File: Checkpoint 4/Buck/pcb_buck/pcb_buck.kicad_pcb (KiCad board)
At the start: 2 copper layers, 90.2 x 37.8 mm, 18 parts, among them J2 Conn_01x04_Socket, M1 IRF530, M2 IRF530, U1 IR2104

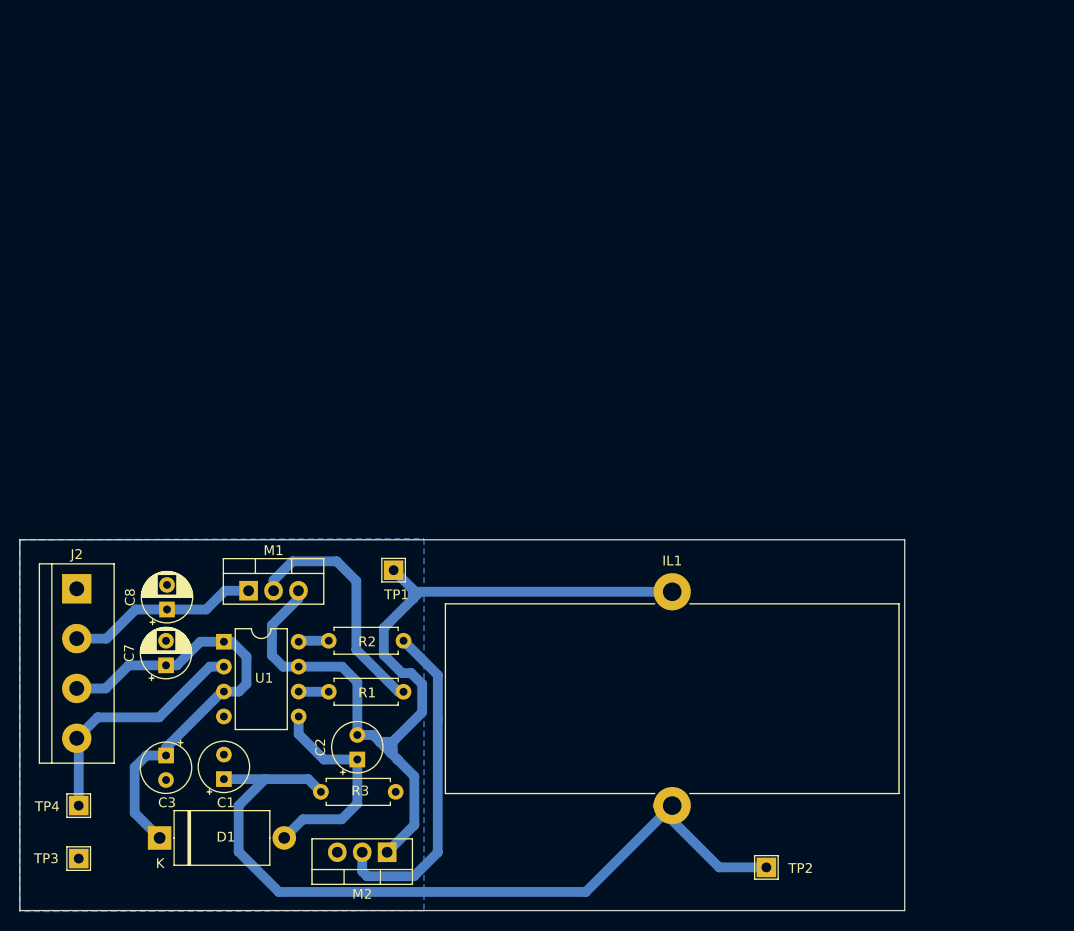
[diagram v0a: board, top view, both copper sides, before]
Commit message: PCB Buck new
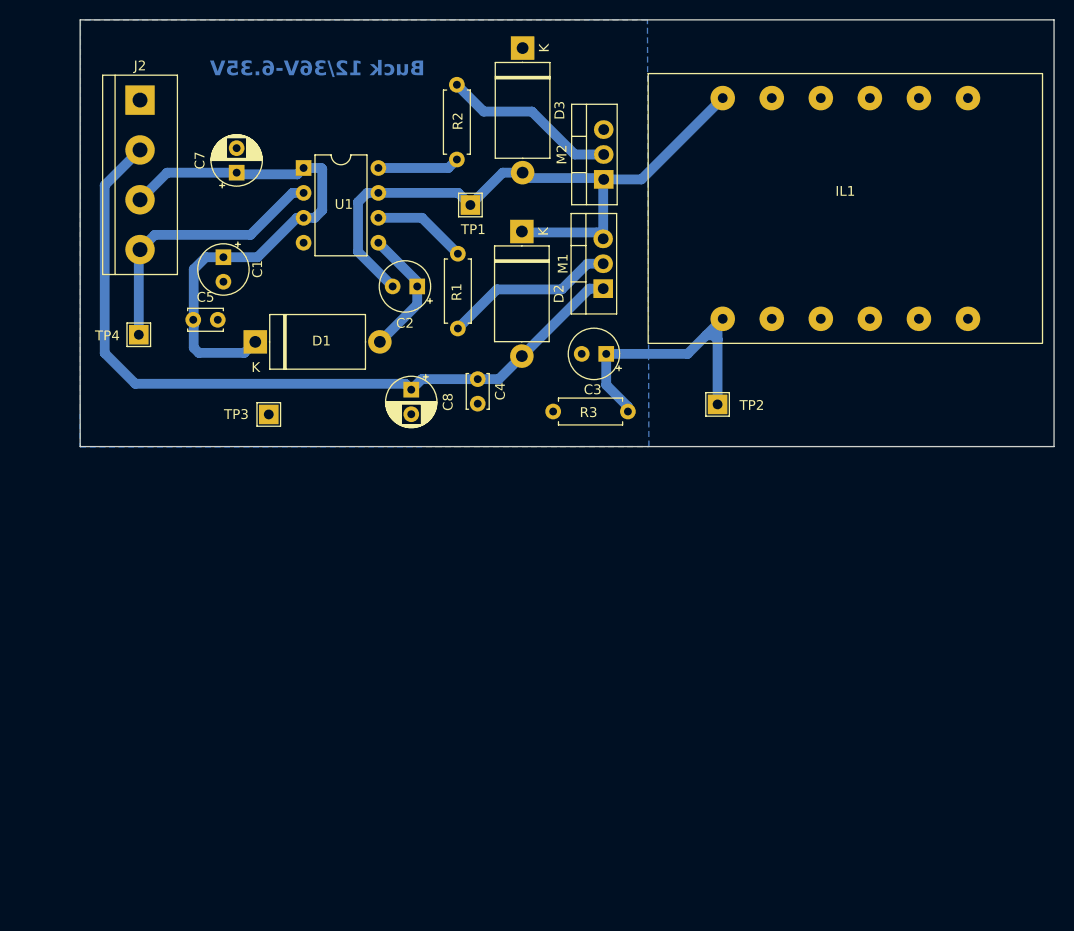
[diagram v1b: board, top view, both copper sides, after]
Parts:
- added C4: 100n, Capacitor_THT:C_Disc_D3.4mm_W2.1mm_P2.50mm, F.Cu at (168.1, 65.5)
- added C5: 100n, Capacitor_THT:C_Disc_D3.4mm_W2.1mm_P2.50mm, F.Cu at (139.1, 59.5)
- added D2: D1n5822rl, Diode_THT:D_DO-27_P12.70mm_Horizontal, F.Cu at (172.6, 50.5)
- added D3: D1n5822rl, Diode_THT:D_DO-27_P12.70mm_Horizontal, F.Cu at (172.7, 31.8)
- IL1: value 500µ -> 700µ; footprint Inductor_THT:L_Toroid_Vertical_L46.0mm_W19.1mm_P21.80mm_Bourns_5700 -> Inductor_EE4012_Vertical:Inductor
- M1, M2: value IRF530 -> IRLZ44N
- moved M2 72.1 mm to (180.9, 45.2), turned to 90 degrees
- moved C3 58.3 mm to (181.2, 63.0), turned to 180 degrees
- moved R2 56.9 mm to (165.9, 35.5), turned to -90 degrees
- moved D1 51.5 mm to (145.4, 61.7)
- moved C1 51.1 mm to (142.2, 53.1)
- moved C7 50.7 mm to (143.5, 44.5)
- moved J2 50.2 mm to (133.7, 37.1)
- moved R3 49.8 mm to (183.4, 68.8), turned to 180 degrees
- moved TP3 49.2 mm to (146.8, 69.1)
- moved U1 49.0 mm to (150.3, 44.0)
- moved C2 48.6 mm to (161.9, 56.1), turned to 180 degrees
- moved TP4 48.4 mm to (133.5, 61.0)
- moved M1 47.5 mm to (180.9, 56.3), turned to 90 degrees
- moved TP2 47.5 mm to (192.5, 68.1)
- moved IL1 42.9 mm to (205.6, 48.1)
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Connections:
- IL1 pad 1: Vd -> Vo
- IL1 pad 2: Vo -> (no net)
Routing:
- net vdd: track 19.7 -> 78.8 mm
- net Vo: track 82.2 -> 30.4 mm
- net Vd: track 94.4 -> 67.9 mm
- net Net-(M2-G): track 33.9 -> 17.9 mm
- net Net-(D1--): track 22.3 -> 13.3 mm
- net vcc: track 46.3 -> 54.5 mm
- net Net-(M1-G): track 24.7 -> 17.5 mm
- net Net-(U1-HO): track 3.08 -> 9.62 mm
- net Net-(U1-LO): track 3.11 -> 8.36 mm
- net pwm: track 25.0 -> 27.8 mm
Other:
- board size 90.2 x 37.8 mm -> 99.3 x 43.5 mm
- board text added: "Buck 12/36V-6.35V"
